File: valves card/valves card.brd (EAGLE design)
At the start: 100 x 80 mm, 68 parts, among them J1 8-1393644-0, J2 TBP02R1-381-14BE, Q1 IRLZ44NSTRLPBF, Q11 IRLZ44NSTRLPBF, Q13 IRLZ44NSTRLPBF, Q15 IRLZ44NSTRLPBF, Q17 IRLZ44NSTRLPBF, Q19 IRLZ44NSTRLPBF, Q21 IRLZ44NSTRLPBF, Q23 IRLZ44NSTRLPBF, Q3 IRLZ44NSTRLPBF, Q5 IRLZ44NSTRLPBF, Q7 IRLZ44NSTRLPBF, Q9 IRLZ44NSTRLPBF, U1 LM2937IMP-10, U10 OR-815, U12 OR-815, U14 OR-815, U16 OR-815, U18 OR-815, U2 OR-815, U20 OR-815, U22 OR-815, U24 OR-815, U4 OR-815, U6 OR-815, U8 OR-815

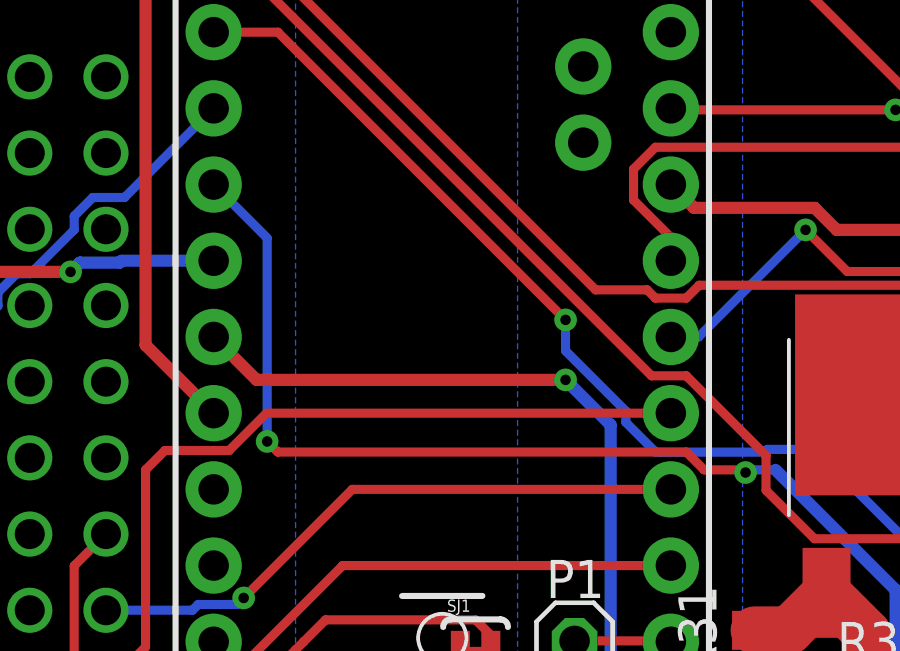
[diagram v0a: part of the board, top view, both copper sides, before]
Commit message: started bom creation
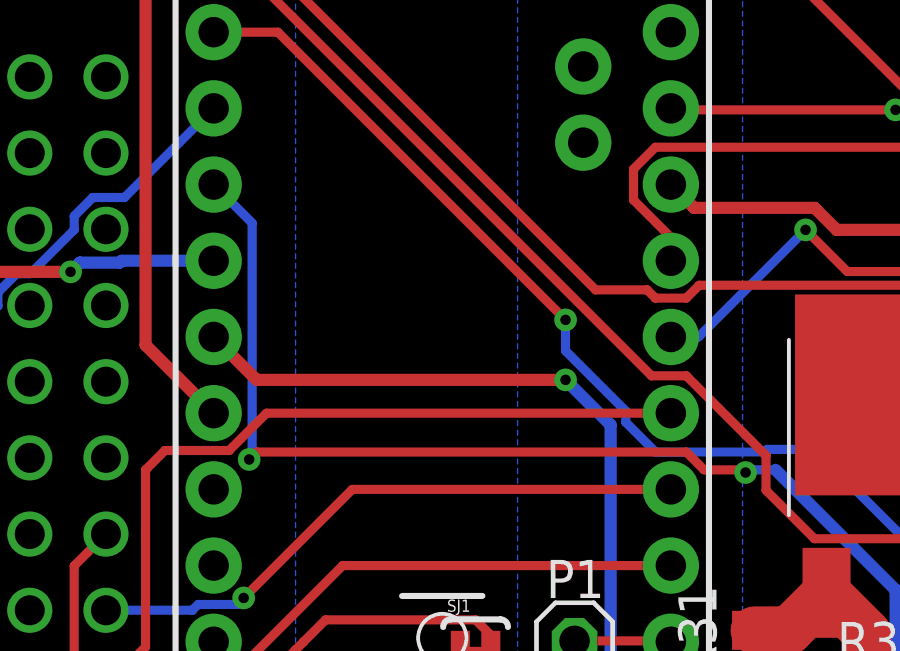
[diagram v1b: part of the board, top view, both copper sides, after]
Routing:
- net SOL3: track 69.5 -> 70.5 mm
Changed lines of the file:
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@@
 <attribute name="DESCRIPTION" value="  Optoisolator Transistor Output 5000Vrms 1 Channel 4-DIP " x="53.5" y="47.8" size="1.778" layer="27" rot="R180" display="off"/>
 <attribute name="MF" value="Everlight" x="53.5" y="47.8" size="1.778" layer="27" rot="R180" display="off"/>
-<attribute name="MP" value="EL817(C)" x="53.5" y="47.8" size="1.778" layer="27" rot="R180" display="off"/>
+<attribute name="MP" value="OR-815" x="53.5" y="47.8" size="1.778" layer="27" rot="R180" display="off"/>
 <attribute name="NAME" x="23.604659375" y="9.19763125" size="1.271159375" layer="25" rot="R180"/>
 <attribute name="PACKAGE" value="DIP-4 Everlight" x="53.5" y="47.8" size="1.778" layer="27" rot="R180" display="off"/>
@@
 <wire x1="37" y1="42" x2="33" y2="46" width="0.4064" layer="16"/>
 <wire x1="37" y1="31" x2="37" y2="42" width="0.4064" layer="16"/>
-<via x="16.053021875" y="46.946978125" extent="1-16" drill="0.35"/>
+<via x="15.453021875" y="46.346978125" extent="1-16" drill="0.35"/>
 <wire x1="30.62013125" y1="46" x2="30.02553125" y2="46.5946" width="0.3048" layer="1"/>
-<wire x1="16.4054" y1="46.5946" x2="16.053021875" y2="46.946978125" width="0.3048" layer="1"/>
-<wire x1="30.02553125" y1="46.5946" x2="16.4054" y2="46.5946" width="0.3048" layer="1"/>
-<wire x1="16.053021875" y1="46.946978125" x2="16.053021875" y2="53.726978125" width="0.3048" layer="16"/>
-<wire x1="16.053021875" y1="53.726978125" x2="14.27" y2="55.51" width="0.3048" layer="16"/>
+<wire x1="15.70064375" y1="46.5946" x2="15.453021875" y2="46.346978125" width="0.3048" layer="1"/>
+<wire x1="30.02553125" y1="46.5946" x2="15.70064375" y2="46.5946" width="0.3048" layer="1"/>
+<wire x1="15.453021875" y1="46.346978125" x2="15.553021875" y2="46.446978125" width="0.3048" layer="16"/>
+<wire x1="15.553021875" y1="54.226978125" x2="15.553021875" y2="46.446978125" width="0.3048" layer="16"/>
+<wire x1="15.553021875" y1="54.226978125" x2="14.27" y2="55.51" width="0.3048" layer="16"/>
 <wire x1="33" y1="46" x2="32.0884" y2="46" width="0.3048" layer="16"/>
 <wire x1="32.0884" y1="46" x2="32" y2="45.9116" width="0.3048" layer="16"/>

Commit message: fixed library attributes for the din41612 connector, fixed git problems
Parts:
- J1: value 8-1393644-0 -> 09231486921; device 8-1393644-0:TE_8-1393644-0 -> din41612_48_pin_board:HARTING_09231486921
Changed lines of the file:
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@@
 </autorouter>
 <elements>
-<element name="J1" library="8-1393644-0" package="TE_8-1393644-0" value="8-1393644-0" x="5.6" y="21" smashed="yes" rot="R270">
+<element name="J1" library="din41612_48_pin_board" package="HARTING_09231486921" value="09231486921" x="5.6" y="21" smashed="yes" rot="R270">
 <attribute name="AVAILABILITY" value="In Stock" x="5.6" y="21" size="1.778" layer="27" rot="R270" display="off"/>
-<attribute name="COMMENT" value="8-1393644-0" x="5.6" y="21" size="1.778" layer="27" rot="R270" display="off"/>
+<attribute name="COMMENT" value="09231486921" x="5.6" y="21" size="1.778" layer="27" rot="R270" display="off"/>
 <attribute name="DESCRIPTION" value=" Conn DIN 41612 M 48 POS 2.54mm Solder RA Thru-Hole Tray " x="5.6" y="21" size="1.778" layer="27" rot="R270" display="off"/>
 <attribute name="EU_ROHS_COMPLIANCE" value="Compliant" x="5.6" y="21" size="1.778" layer="27" rot="R270" display="off"/>
-<attribute name="MF" value="TE Connectivity" x="5.6" y="21" size="1.778" layer="27" rot="R270" display="off"/>
-<attribute name="MP" value="8-1393644-0" x="5.6" y="21" size="1.778" layer="27" rot="R270" display="off"/>
+<attribute name="MF" value="HARTING" x="5.6" y="21" size="1.778" layer="27" rot="R270" display="off"/>
+<attribute name="MP" value="09231486921" x="5.6" y="21" size="1.778" layer="27" rot="R270" display="off"/>
 <attribute name="NAME" x="12.605" y="67.73" size="1.27" layer="25" rot="R270"/>
 <attribute name="PACKAGE" value="None" x="5.6" y="21" size="1.778" layer="27" rot="R270" display="off"/>
-<attribute name="PRICE" value="None" x="5.6" y="21" size="1.778" layer="27" rot="R270" display="off"/>
-<attribute name="PURCHASE-URL" value="https://pricing.snapeda.com/search/part/8-1393644-0/?ref=eda" x="5.6" y="21" size="1.778" layer="27" rot="R270" display="off"/>
+<attribute name="PRICE" value="6$" x="5.6" y="21" size="1.778" layer="27" rot="R270" display="off"/>
+<attribute name="PURCHASE-URL-DIGIKEY" value="https://www.digikey.ca/en/products/detail/harting/09231486921/3180439" x="5.6" y="21" size="1.778" layer="27" rot="R270" display="off"/>
 <attribute name="VALUE" x="-8.59" y="67.73" size="1.27" layer="27" rot="R270"/>
 </element>
